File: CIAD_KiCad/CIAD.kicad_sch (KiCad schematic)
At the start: 25 parts, among them J2 Conn_01x08, SW1 SW_Push, SW10 SW_Push, SW11 SW_Push, SW2 SW_Push, SW3 SW_Push, SW4 SW_Push, SW5 SW_Push, SW6 SW_Push, SW7 SW_Push, SW8 SW_Push, SW9 SW_Push, U1 74HC595, U2 74HC595

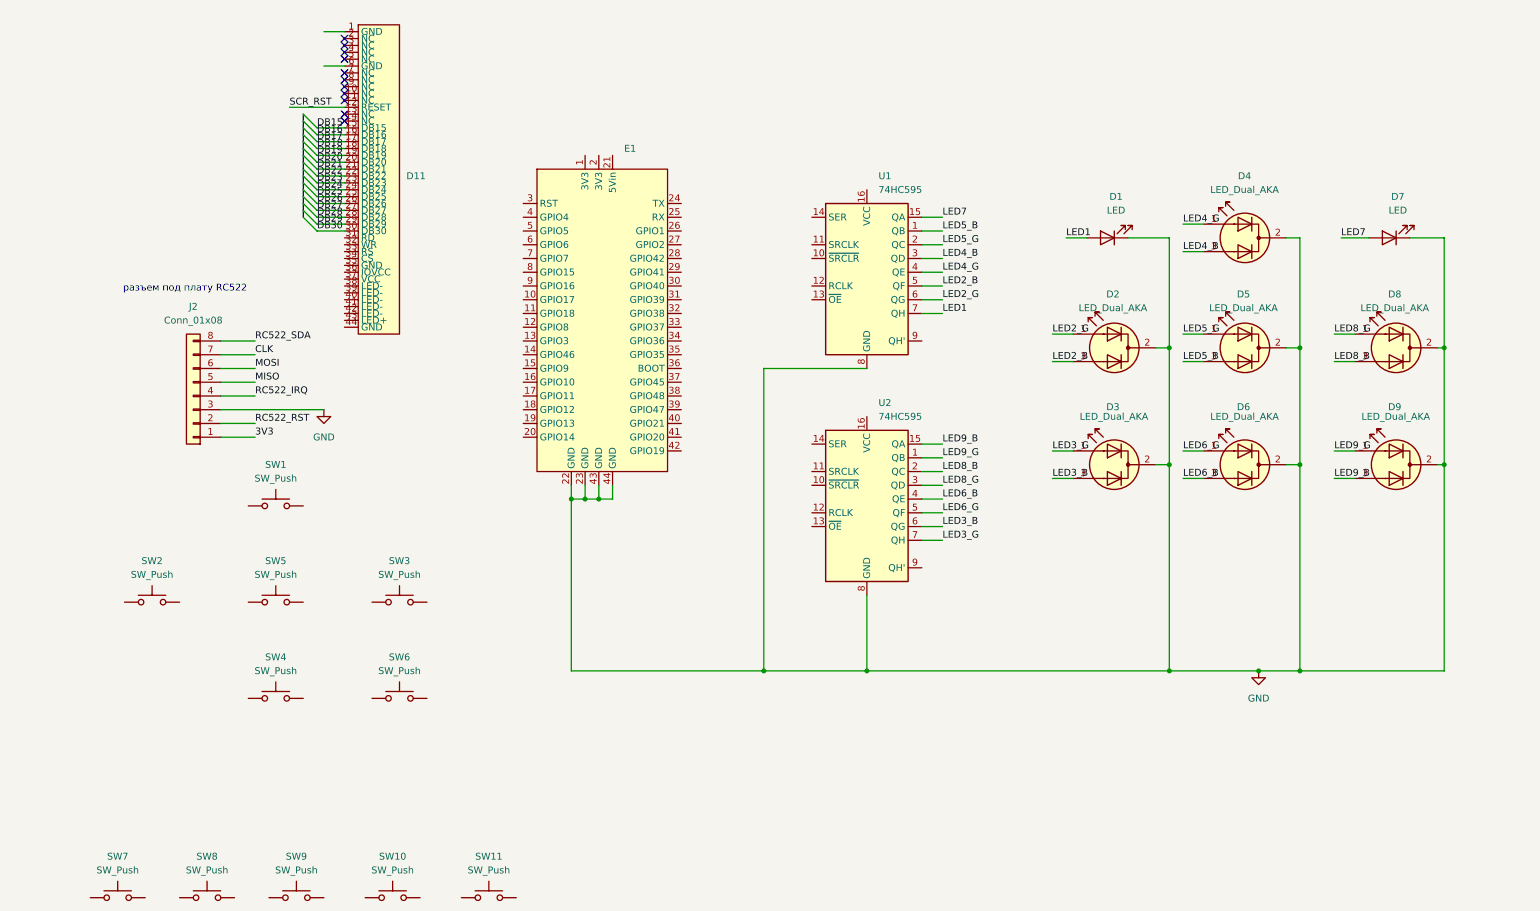
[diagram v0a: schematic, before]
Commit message: small updates to hardware
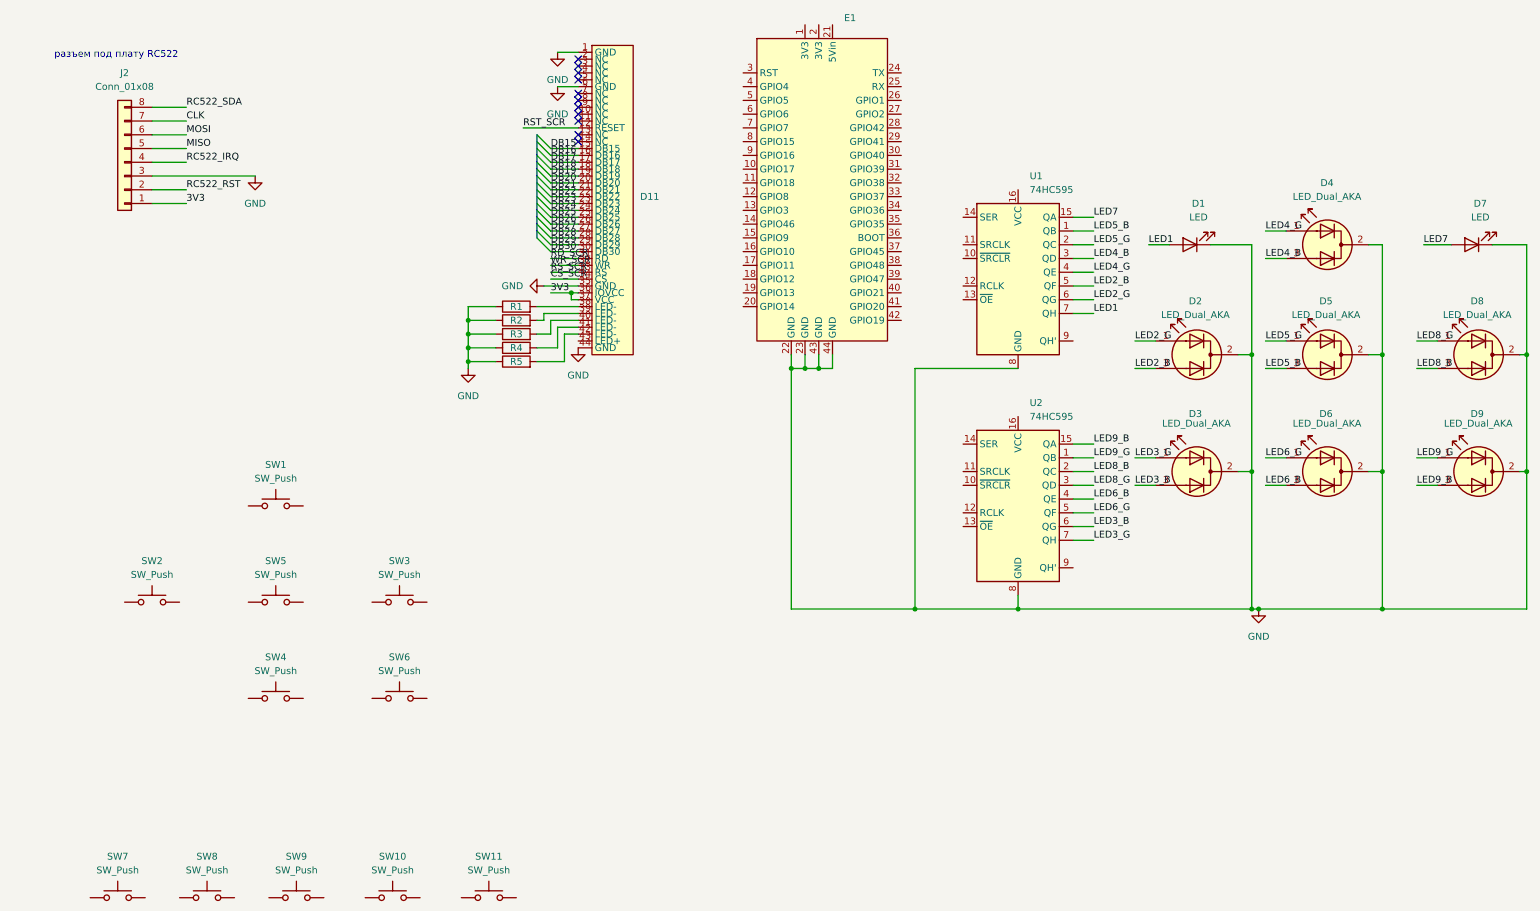
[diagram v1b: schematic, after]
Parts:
- added R1, R2, R3, R4, R5: R, symbol Device:R
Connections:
- net 3V3: now also D11.36 (IOVCC), D11.37 (VCC)
- net GND: now also D11.1 (GND), D11.35 (GND), D11.44 (GND), D11.6 (GND), R1.1, R2.1, R3.1, R4.1, R5.1
- net RD_SCR: now reaches D11.31 (RD)
- net WR_SCR: now reaches D11.32 (WR)
- net RS_SCR: now reaches D11.33 (RS)
- net CS_SCR: now reaches D11.34 (CS)
- net at D11.38 (LED-): now also R1.2
- net at D11.39 (LED-): now also R2.2
- net at D11.40 (LED-): now also R3.2
- net at D11.41 (LED-): now also R4.2
- net at D11.42 (LED-): now also R5.2
- net SCR_RST renamed RST_SCR
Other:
- moved on the sheet: D1, D11, D2, D3, D4, D5, D6, D7, D8, D9, E1, J2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
